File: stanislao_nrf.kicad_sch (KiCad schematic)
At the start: 13 parts, among them J1 JST_HX_S6B, J2 Conn_01x02, J3 Conn_01x02, J4 Conn_01x02, J5 Conn_01x02, Q1 BTS4140N, Q2 BSP89, U1 NRF52840-DONGLE, U2 TPSM265R1

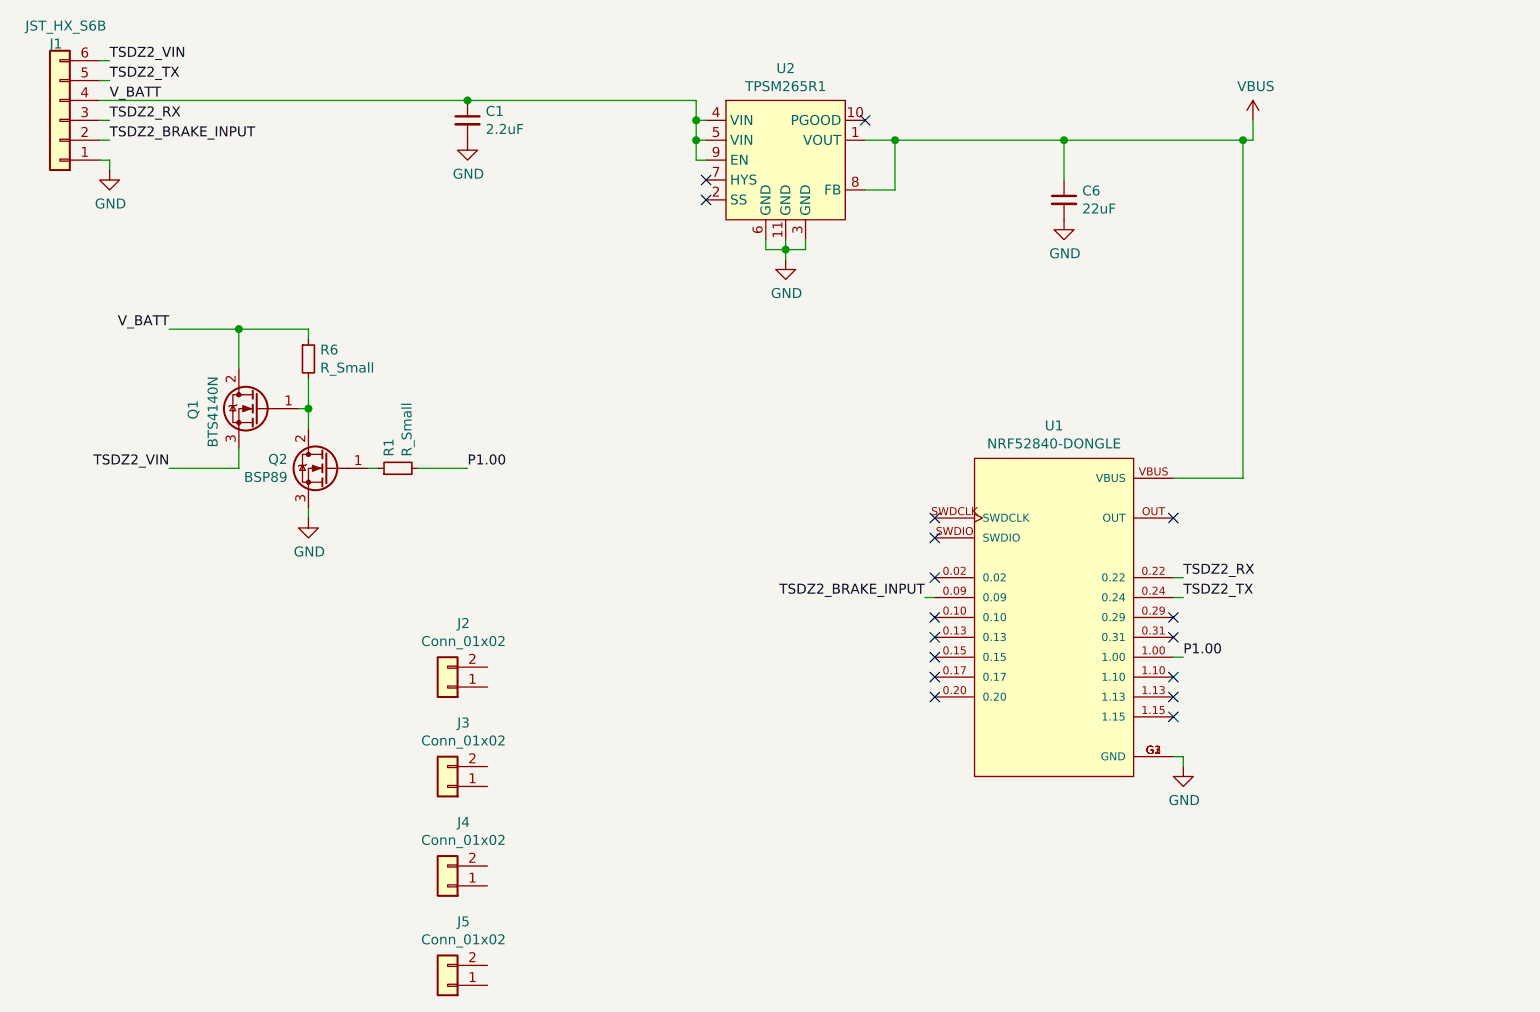
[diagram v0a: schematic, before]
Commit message: Awaiting for logo
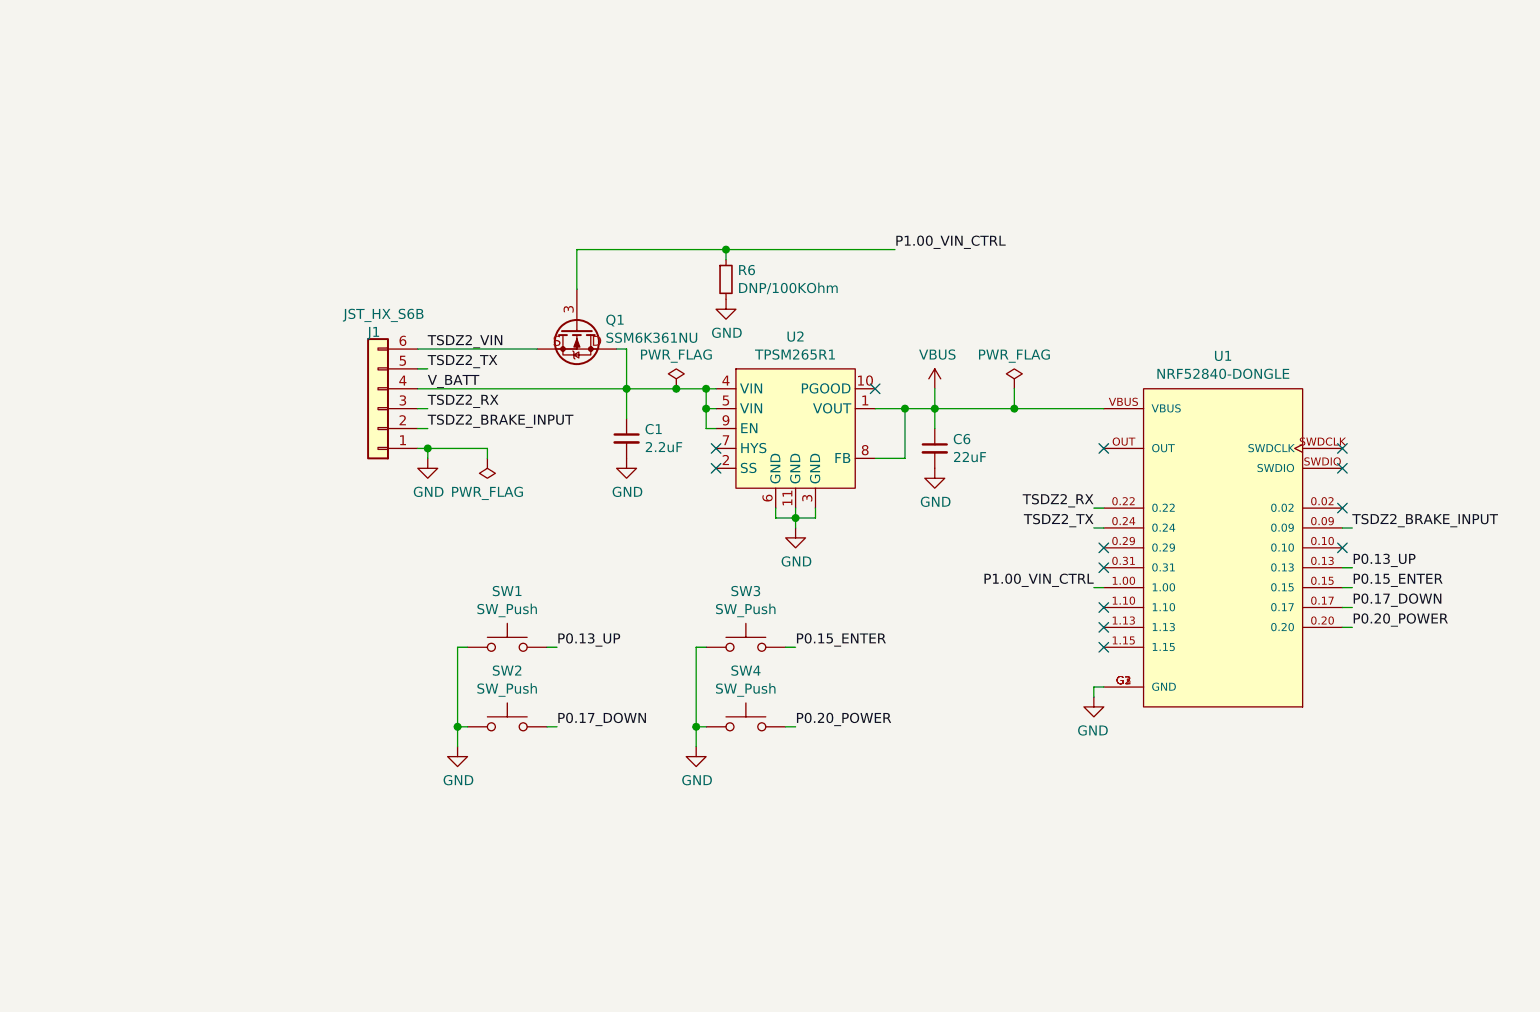
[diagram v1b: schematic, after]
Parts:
- removed J2, J3, J4, J5: Conn_01x02, Connector_JST:JST_XH_B2B-XH-A_1x02_P2.50mm_Vertical, symbol Connector_Generic:Conn_01x02
- removed Q1: BTS4140N, Package_TO_SOT_SMD:SOT-223-3_TabPin2, symbol Transistor_FET:BSP89
- removed Q2: BSP89, Package_TO_SOT_SMD:SOT-223-3_TabPin2, symbol Transistor_FET:BSP89
- removed R1: R_Small, Resistor_SMD:R_0603_1608Metric, symbol Device:R_Small
- added Q1: SSM6J507NU, footprints:UDFN6B, symbol SSM6J507NU:SSM6J507NU
- added SW1, SW2, SW3, SW4: SW_Push, Connector_JST:JST_XH_B2B-XH-A_1x02_P2.50mm_Vertical, symbol Switch:SW_Push
- R6: value R_Small -> DNP/100KOhm
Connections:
- net GND: now also R6.2, SW1.1, SW2.1, SW3.1, SW4.1
- net TSDZ2_VIN: now also Q1.4 (S), Q1.S
- net V_BATT: now also Q1.1 (D), Q1.2 (D), Q1.5 (D), Q1.6 (D), Q1.D; no longer R6.1
- net P0.13_UP: now reaches U1.0.13
- net P0.13_UP: now also SW1.2
- net P0.15_ENTER: now reaches U1.0.15
- net P0.15_ENTER: now also SW3.2
- net P0.17_DOWN: now reaches U1.0.17
- net P0.17_DOWN: now also SW2.2
- net P0.20_POWER: now reaches U1.0.20
- net P0.20_POWER: now also SW4.2
- net P1.00 renamed P1.00_VIN_CTRL
- net P1.00_VIN_CTRL: now also R6.1, Q1.3 (G)
- no-connect marks 17 -> 13
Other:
- moved on the sheet: C1, C6, J1, R6, U1, U2
